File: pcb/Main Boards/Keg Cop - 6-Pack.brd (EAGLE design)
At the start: 29.9 x 43.2 mm, 3 parts, among them X1 RJ45-8X, X2 RJ45-8X

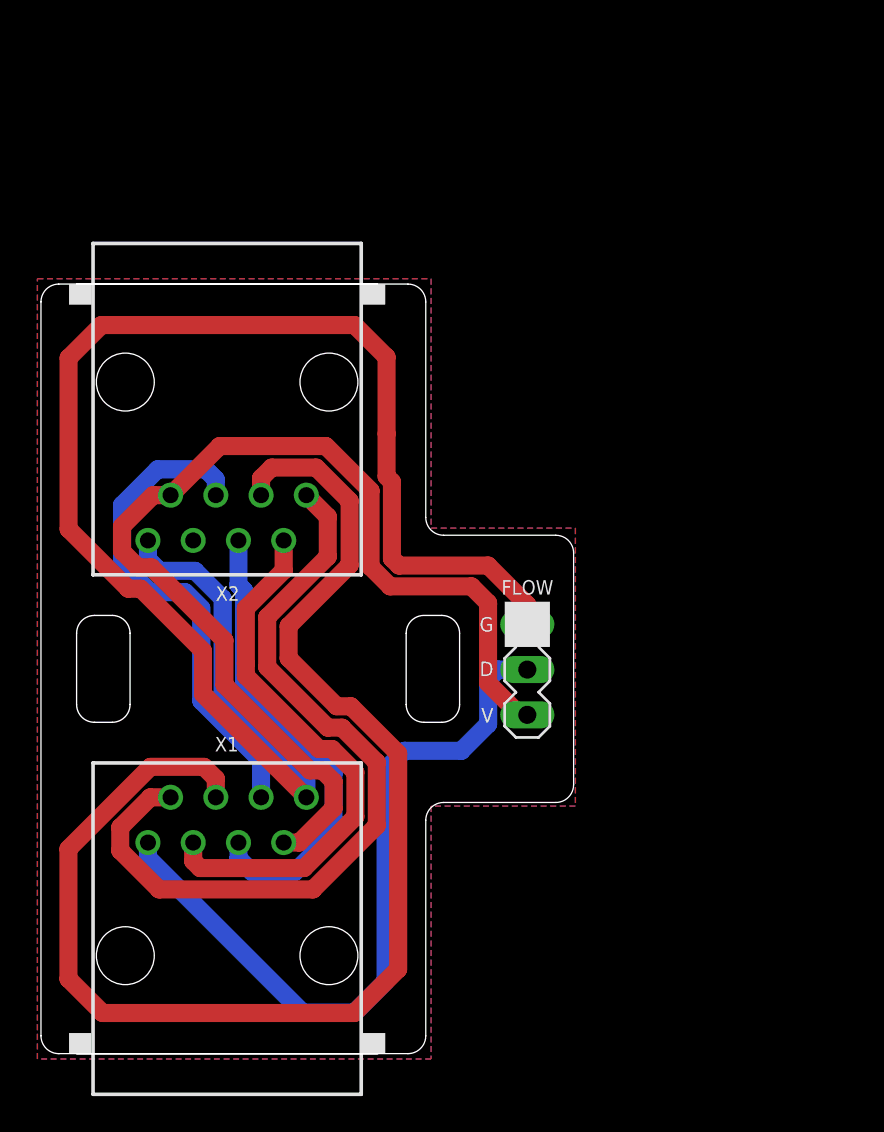
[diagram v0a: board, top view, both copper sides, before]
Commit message: Rename files
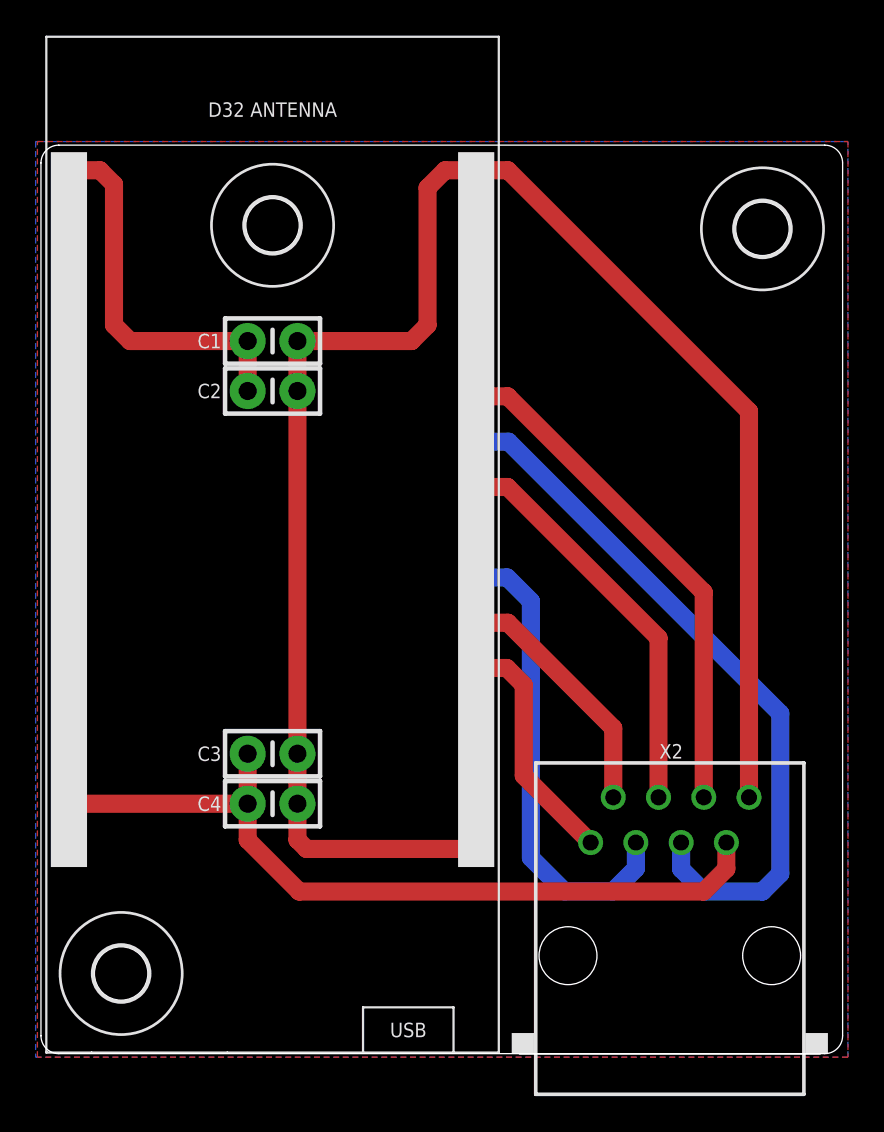
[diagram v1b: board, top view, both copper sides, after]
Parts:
- removed FLOW: 3-PIN, Donnie:HDR-3_VERT
- removed X1: RJ45-8X, con-tycoelectronics:RJ45-NO-SHIELD
- added C1, C3: 0.1μF, Donnie:CAP_PTH-2.54
- added C2, C4: 1.0μF, Donnie:CAP_PTH-2.54
- added D32: Lolin D32, Donnie:D32_NO_BATT
- added U$1, U$2, U$3: (no value), holes:3,0
- moved X2 40.7 mm to (35.3, 5.50), turned to 0 degrees
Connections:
- removed net FLOW: FLOW.2, X1.1
- removed net N$1: X1.2, X2.1
- removed net N$2: X1.3, X2.2
- removed net N$3: X1.4, X2.3
- removed net N$5: X1.5, X2.4
- removed net N$7: X1.6, X2.5
- new net KEG1: D32.IO4, X2.1
- new net KEG2: D32.IO16, X2.2
- new net KEG3: D32.IO17, X2.3
- new net KEG4: D32.IO18, X2.4
- new net KEG5: D32.IO19, X2.5
- new net KEG6: D32.IO21, X2.6
- new net VCC: C1.1, C2.1, D32.VCC
- net 5V: now also C3.1, C4.1, D32.VBUS; no longer FLOW.3, X1.7
- net GND: now also C1.2, C2.2, C3.2, C4.2, D32.GND, D32.GND2; no longer FLOW.1, X1.8
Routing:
- net N$3: track 76.8 -> 0.00 mm
- net N$1: track 45.1 -> 0.00 mm
- net FLOW: track 42.2 -> 0.00 mm
- net KEG5: track 0.00 -> 40.4 mm
- net N$2: track 30.9 -> 0.00 mm
- net KEG6: track 0.00 -> 28.8 mm
- net N$7: track 28.0 -> 0.00 mm
- net KEG3: track 0.00 -> 26.7 mm
- net N$5: track 26.1 -> 0.00 mm
- net KEG4: track 0.00 -> 22.7 mm
- net VCC: track 0.00 -> 21.4 mm
- net 5V: track 61.2 -> 44.9 mm
- net KEG2: track 0.00 -> 14.0 mm
- net KEG1: track 0.00 -> 13.5 mm
- net GND: track 90.4 -> 99.3 mm
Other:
- board size 29.9 x 43.2 mm -> 45 x 51 mm
- board text added: "1 - KEG1 2 - KEG2 3 - KEG3 4 - KEG4"
- board text added: "5 - KEG5 6 - KEG6 7 - KEG7 8 - KEG8"
- board text removed: "D"
- board text removed: "G"
- board text removed: "V"
